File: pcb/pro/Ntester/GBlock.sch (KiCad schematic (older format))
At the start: 20 parts, among them U2 LT6233, U3 LT6233

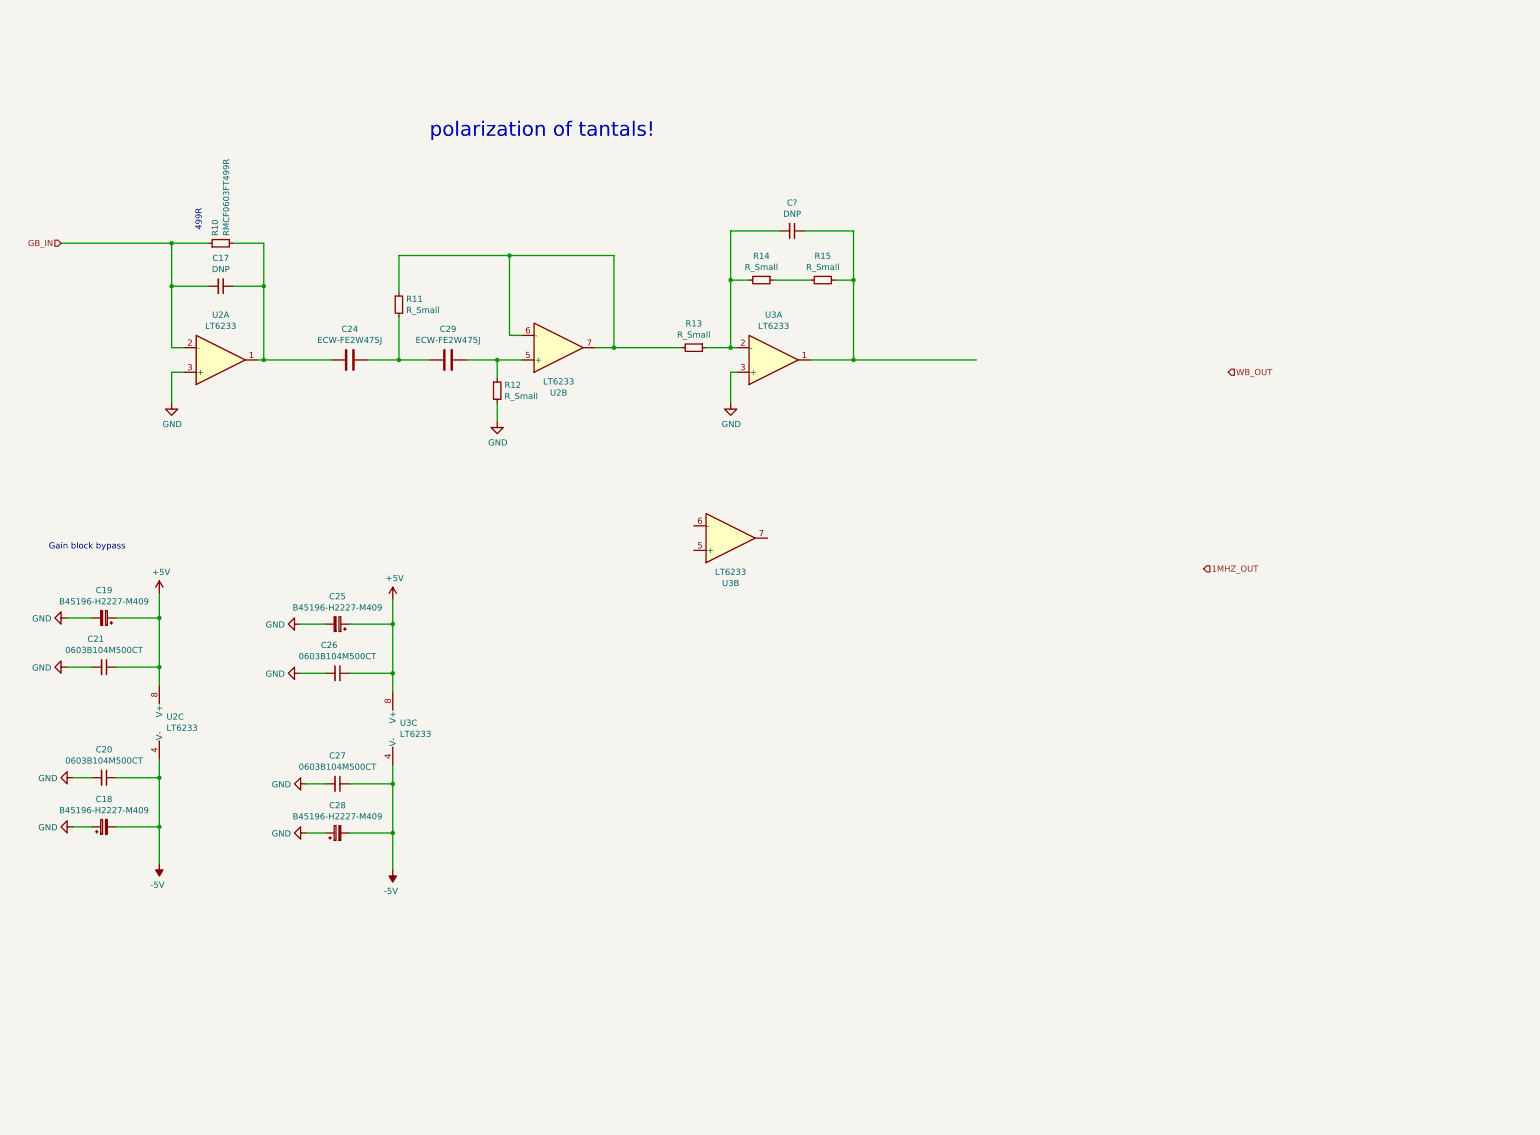
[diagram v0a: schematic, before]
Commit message: " alomost" finalized layout
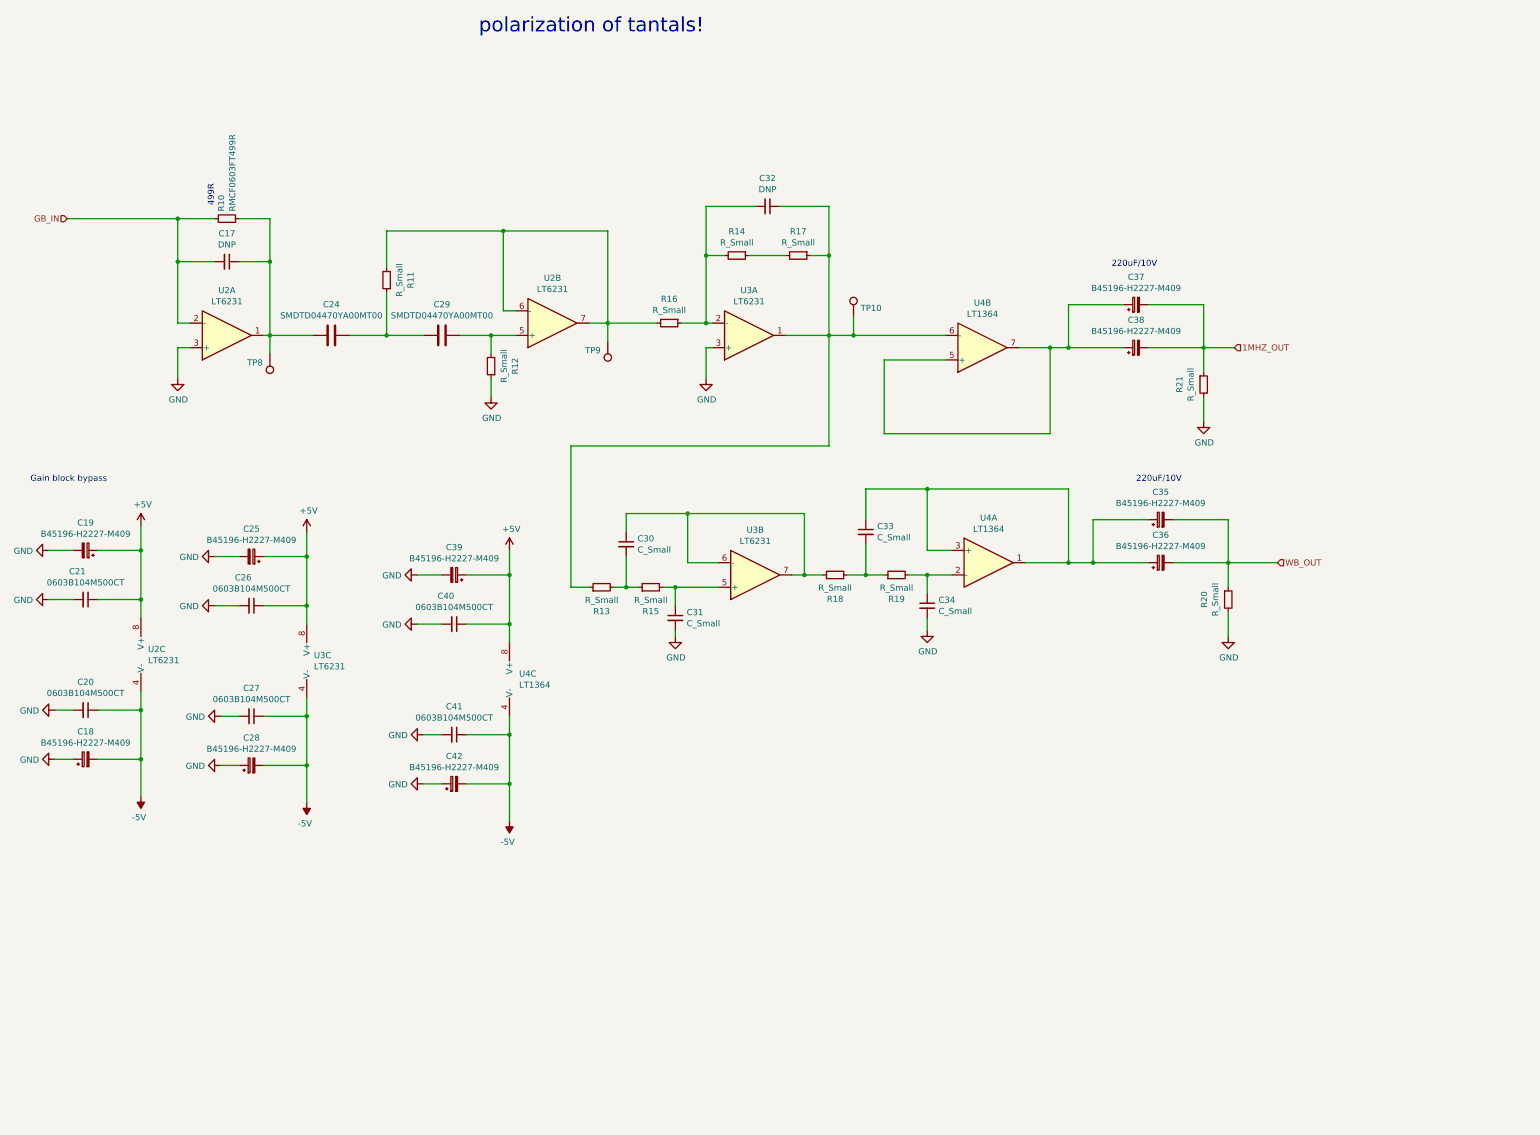
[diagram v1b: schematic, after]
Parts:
- removed U2, U3: LT6233, symbol Amplifier_Operational:LT6233
- added C30, C31, C33, C34: C_Small, Capacitor_SMD:C_0603_1608Metric, symbol Device:C_Small
- added C35, C36, C37, C38, C39, C42: B45196-H2227-M409, Capacitor_Tantalum_SMD:CP_EIA-7343-31_Kemet-D, symbol Device:CP_Small
- added C40, C41: 0603B104M500CT, Resistor_SMD:R_0603_1608Metric, symbol Device:C_Small
- added R16, R17, R18, R19: R_Small, Resistor_SMD:R_0603_1608Metric, symbol Device:R_Small
- added R20, R21: R_Small, Resistor_SMD:R_1206_3216Metric, symbol Device:R_Small
- added TP10, TP8, TP9: TestPoint, TestPoint:TestPoint_THTPad_D1.0mm_Drill0.5mm, symbol Connector:TestPoint
- added U2, U3: LT6231, Ntester:SOIC-8-LINEAR, symbol Ntester_additional:LT6231
- added U4: LT1364, Ntester:SOIC-8-LINEAR, symbol Ntester_additional:LT1364
- C24, C29: value ECW-FE2W475J -> SMDTD04470YA00MT00; footprint Capacitor_THT:C_Rect_L26.5mm_W11.5mm_P22.50mm_MKS4 -> Ntester:CAP-6054-SMDTD04470YA00MT00
- R10: value RMCF0603FT499R -> RMCF0603FT499R
- R11, R12, R13, R14, R15: footprint (none) -> Resistor_SMD:R_0603_1608Metric
- gave numbers to parts that had none: 1
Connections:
- net +5V: now also C39.1, C40.1, U2.8 (V+), U3.8 (V+), U4.8 (V+)
- net -5V: now also C41.1, C42.2, U2.4 (V-), U3.4 (V-), U4.4 (V-)
- net 1MHZ_OUT: now also C37.2, C38.2, R21.1
- net GB_IN: now also U2.2 (-)
- net GND: now also R12.1, C31.2, C34.2, C39.2, C40.2, C41.2, C42.1, R20.2, R21.2, U2.3 (+), U3.3 (+); no longer R12.2
- net WB_OUT: now also C35.2, C36.2, R20.1
- net at C24.1, C29.2: now also R11.1; no longer R11.2
- net at C17.1, C24.2, R10.2: now also TP8.1, U2.1
- net at C29.1: now also R12.2, U2.5 (+); no longer R12.1
- net at R13.2: now also R15.1, C30.2; no longer R11.1
- net at C32.1: now also R13.1, R17.1, TP10.1, U3.1, U4.6 (-); no longer R15.1
- net at C32.2, R14.2: now also R16.1, U3.2 (-); no longer R13.1
- net at R15.2: now also C31.1, U3.5 (+); no longer R14.1
- new net: R11.2, R16.2, TP9.1, U2.6 (-), U2.7
- new net: C33.1, C35.1, C36.1, U4.1, U4.3 (+)
- new net: C34.1, R19.2, U4.2 (-)
- new net: C37.1, C38.1, U4.5 (+), U4.7
- new net: C30.1, R18.1, U3.6 (-), U3.7
- new net: R14.1, R17.2
- new net: C33.2, R18.2, R19.1
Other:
- note added: "220uF/10V"
- moved on the sheet: C17, C18, C19, C20, C21, C24, C25, C26, C27, C28, C29, C32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

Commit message: layout finalized
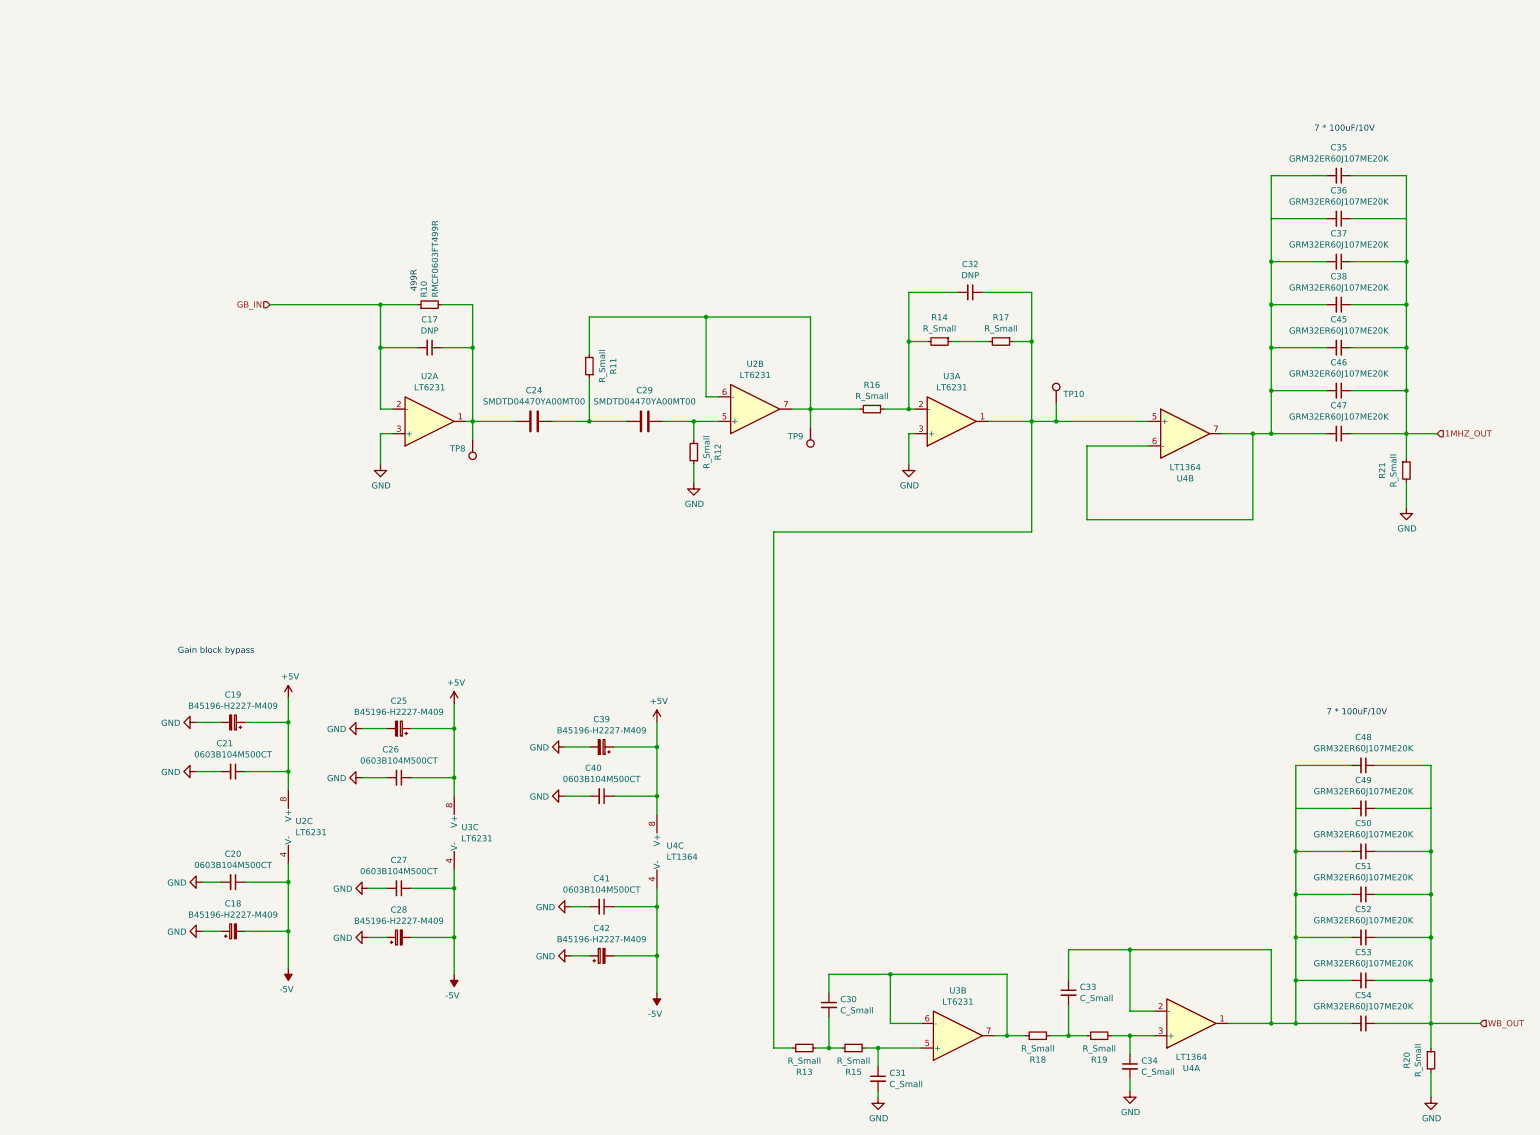
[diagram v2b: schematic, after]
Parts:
- removed C35, C36, C37, C38: B45196-H2227-M409, Capacitor_Tantalum_SMD:CP_EIA-7343-31_Kemet-D, symbol Device:CP_Small
- added C35, C36, C37, C38, C45, C46, C47, C48, C49, C50, C51, C52, C53, C54: GRM32ER60J107ME20K, Capacitor_SMD:C_1210_3225Metric, symbol Device:C_Small
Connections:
- net 1MHZ_OUT: now also C35.1, C36.1, C37.1, C38.1, C45.1, C46.1, C47.1
- net WB_OUT: now also C48.1, C49.1, C50.1, C51.1, C52.1, C53.1, C54.1
- net at C33.1, U4.1: now also U4.2 (-), C48.2, C49.2, C50.2, C51.2, C52.2, C53.2, C54.2; no longer U4.3 (+)
- net at C34.1, R19.2: now also U4.3 (+); no longer U4.2 (-)
- net at U4.5 (+): now also C32.1, R13.1, R17.1, TP10.1, U3.1; no longer U4.7
- new net: C35.2, C36.2, C37.2, C38.2, C45.2, C46.2, C47.2, U4.6 (-), U4.7
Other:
- note added: "7 * 100uF/10V"
- note removed: "220uF/10V"
- note removed: "polarization of tantals!"
- moved on the sheet: C17, C18, C19, C20, C21, C24, C25, C26, C27, C28, C29, C30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
